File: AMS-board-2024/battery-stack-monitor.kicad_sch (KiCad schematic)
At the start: 8 parts, among them U23 LM25180-Q1, U24 LTC2949

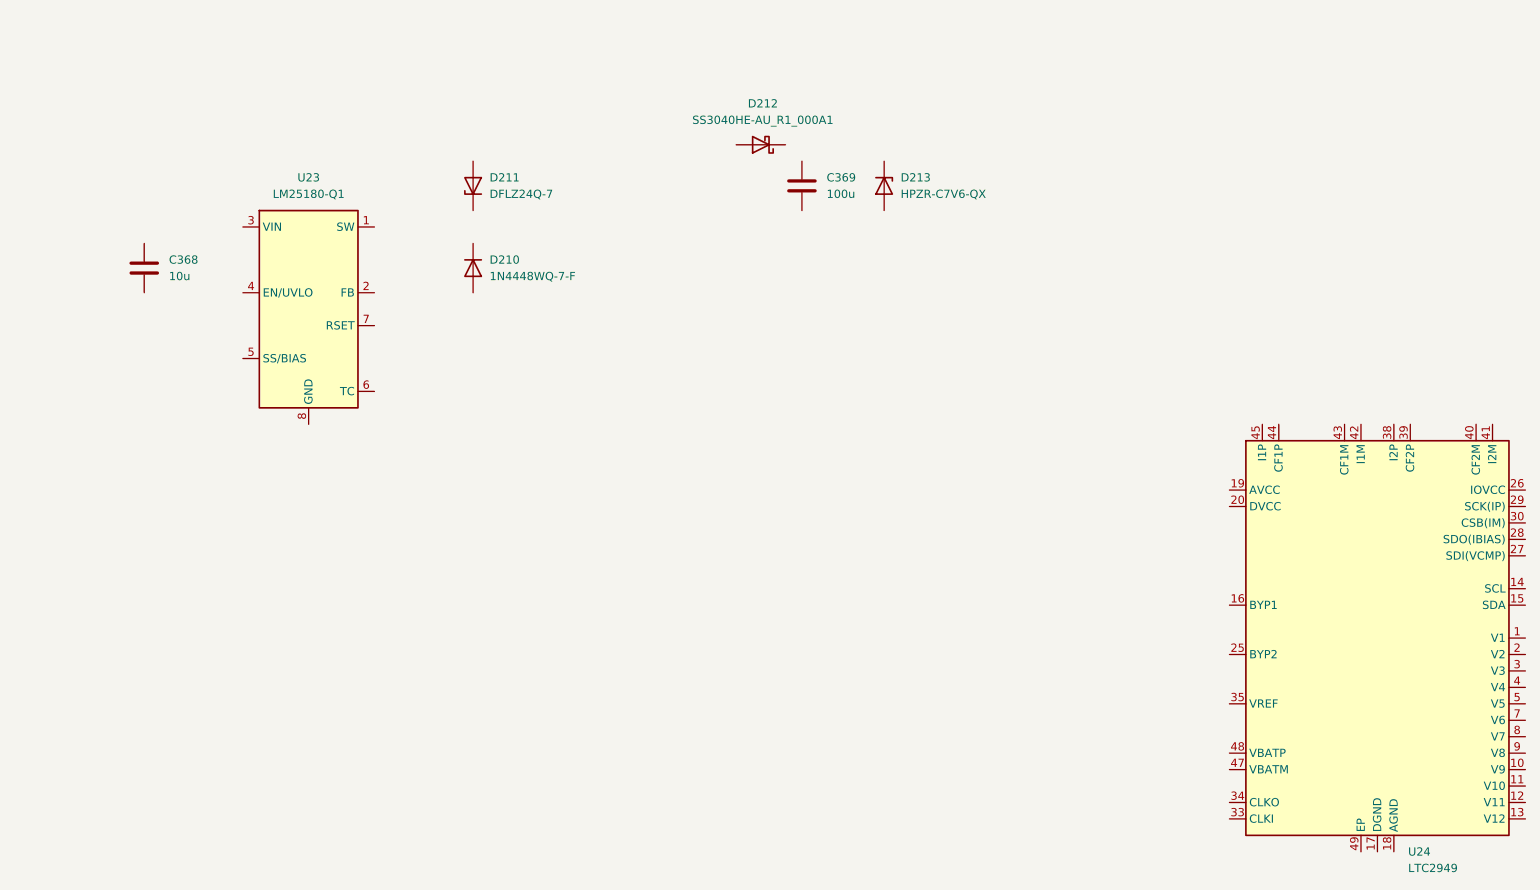
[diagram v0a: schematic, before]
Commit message: 絶縁電源作成
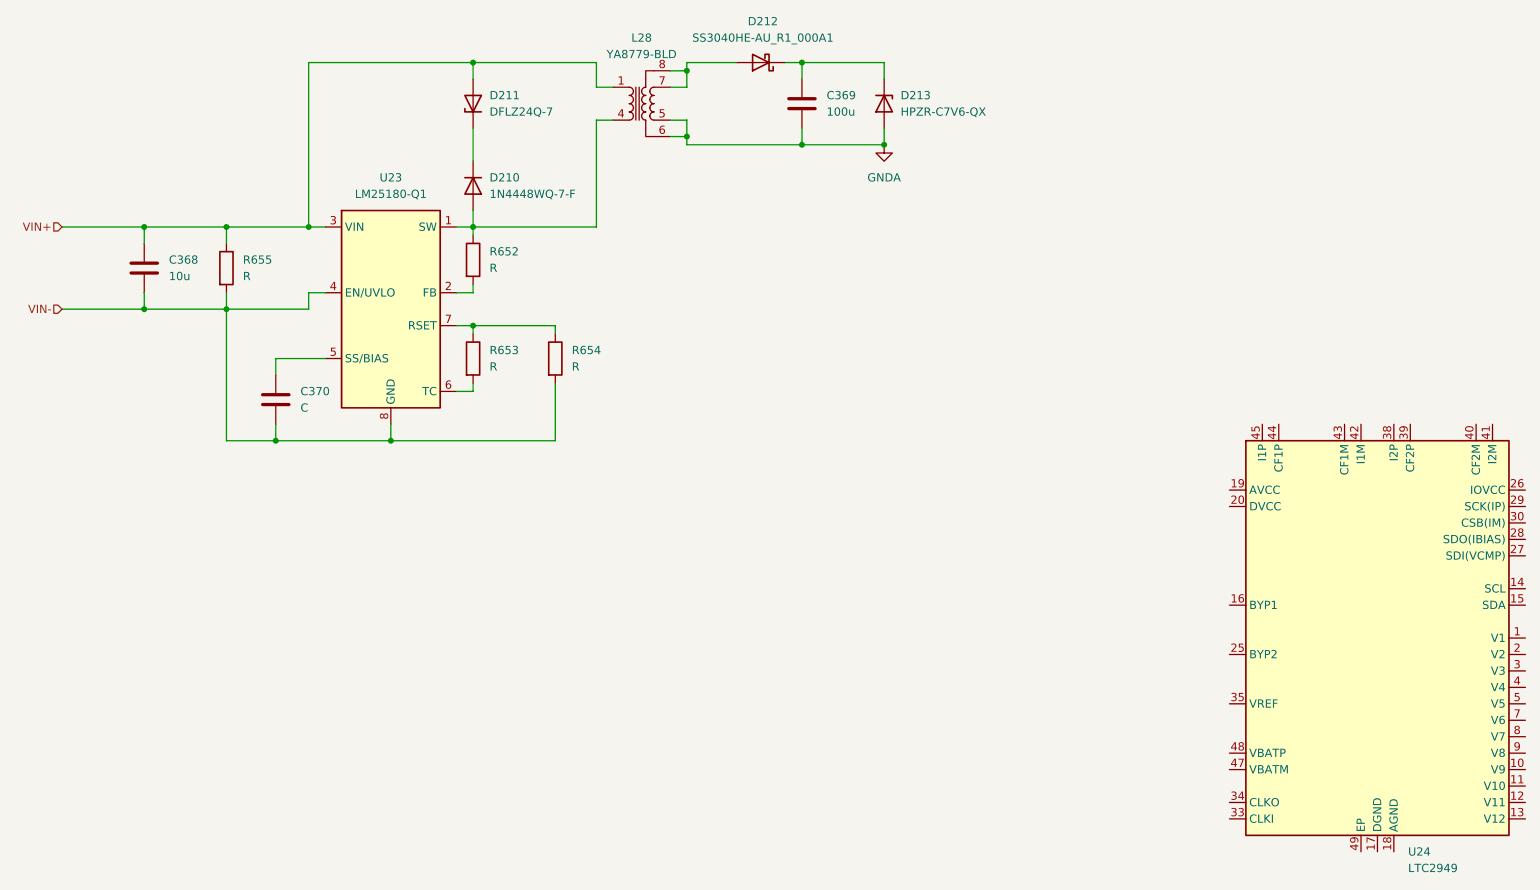
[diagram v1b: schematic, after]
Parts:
- added C370: C, symbol Device:C
- added L28: YA8779-BLD, ProjectEV:Transformer_YA8779-BLD, symbol ProjectEV:Transformer_YA8779
- added R652, R653, R654, R655: R, symbol Device:R
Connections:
- net at U23.1 (SW): now also D210.2 (A), L28.4, R652.1
- net at U23.2 (FB): now also R652.2
- net VIN+: now reaches U23.3 (VIN)
- net VIN+: now also C368.1, D211.2 (A), L28.1, R655.1
- net VIN-: now reaches U23.4 (EN/UVLO)
- net VIN-: now also C368.2, U23.8 (GND), U23.9 (DAP), C370.2, R654.2, R655.2
- net at U23.5 (SS/BIAS): now also C370.1
- net at U23.6 (TC): now also R653.2
- net at U23.7 (RSET): now also R653.1, R654.1
- net at C369.1: now also D212.1 (K), D213.1 (K)
- net GNDA: now reaches C369.2
- net GNDA: now also D213.2 (A), L28.5, L28.6
- net at D211.1 (K): now also D210.1 (K)
- net at D212.2 (A): now also L28.7, L28.8
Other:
- moved on the sheet: C369, D210, D211, D212, D213, U23
